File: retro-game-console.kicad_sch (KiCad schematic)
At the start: 16 parts, among them SW1 SW_Push, SW2 SW_Push, U1 ESP32-DevKitC, U2 Battery_shield_v3, U3 Micro_SD_card_adapter, U4 MAX98357A_Breakout, U5 LCD_ILI9341, U6 74HC165

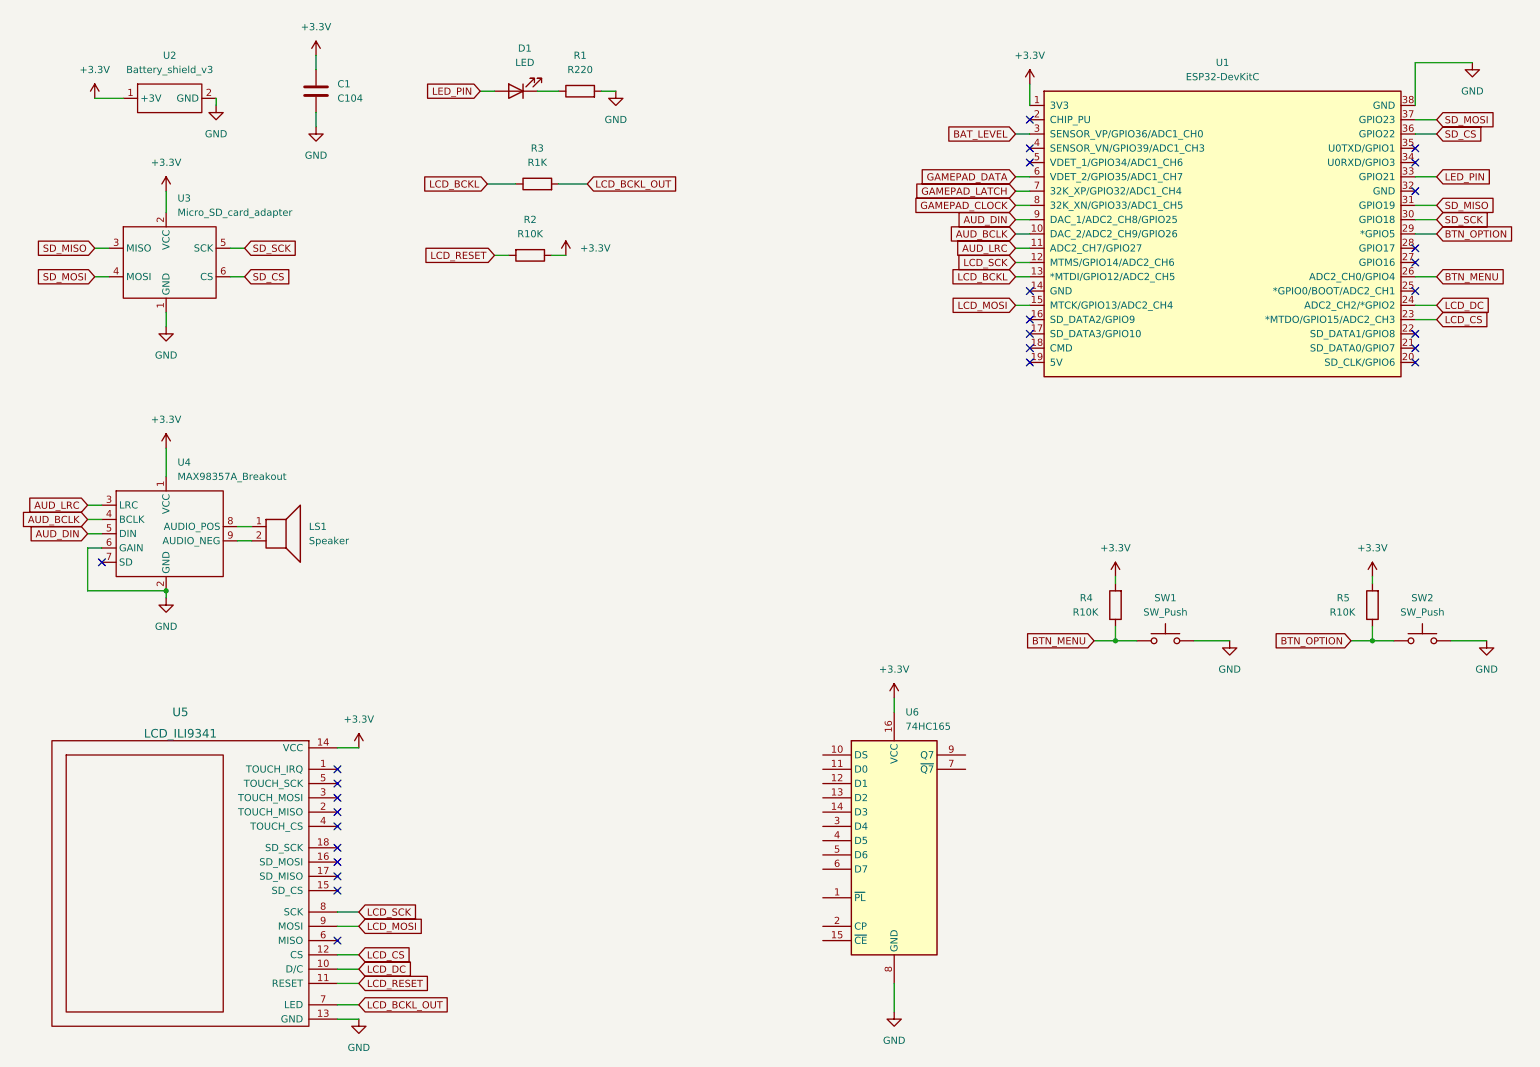
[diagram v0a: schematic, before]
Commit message: Schema done
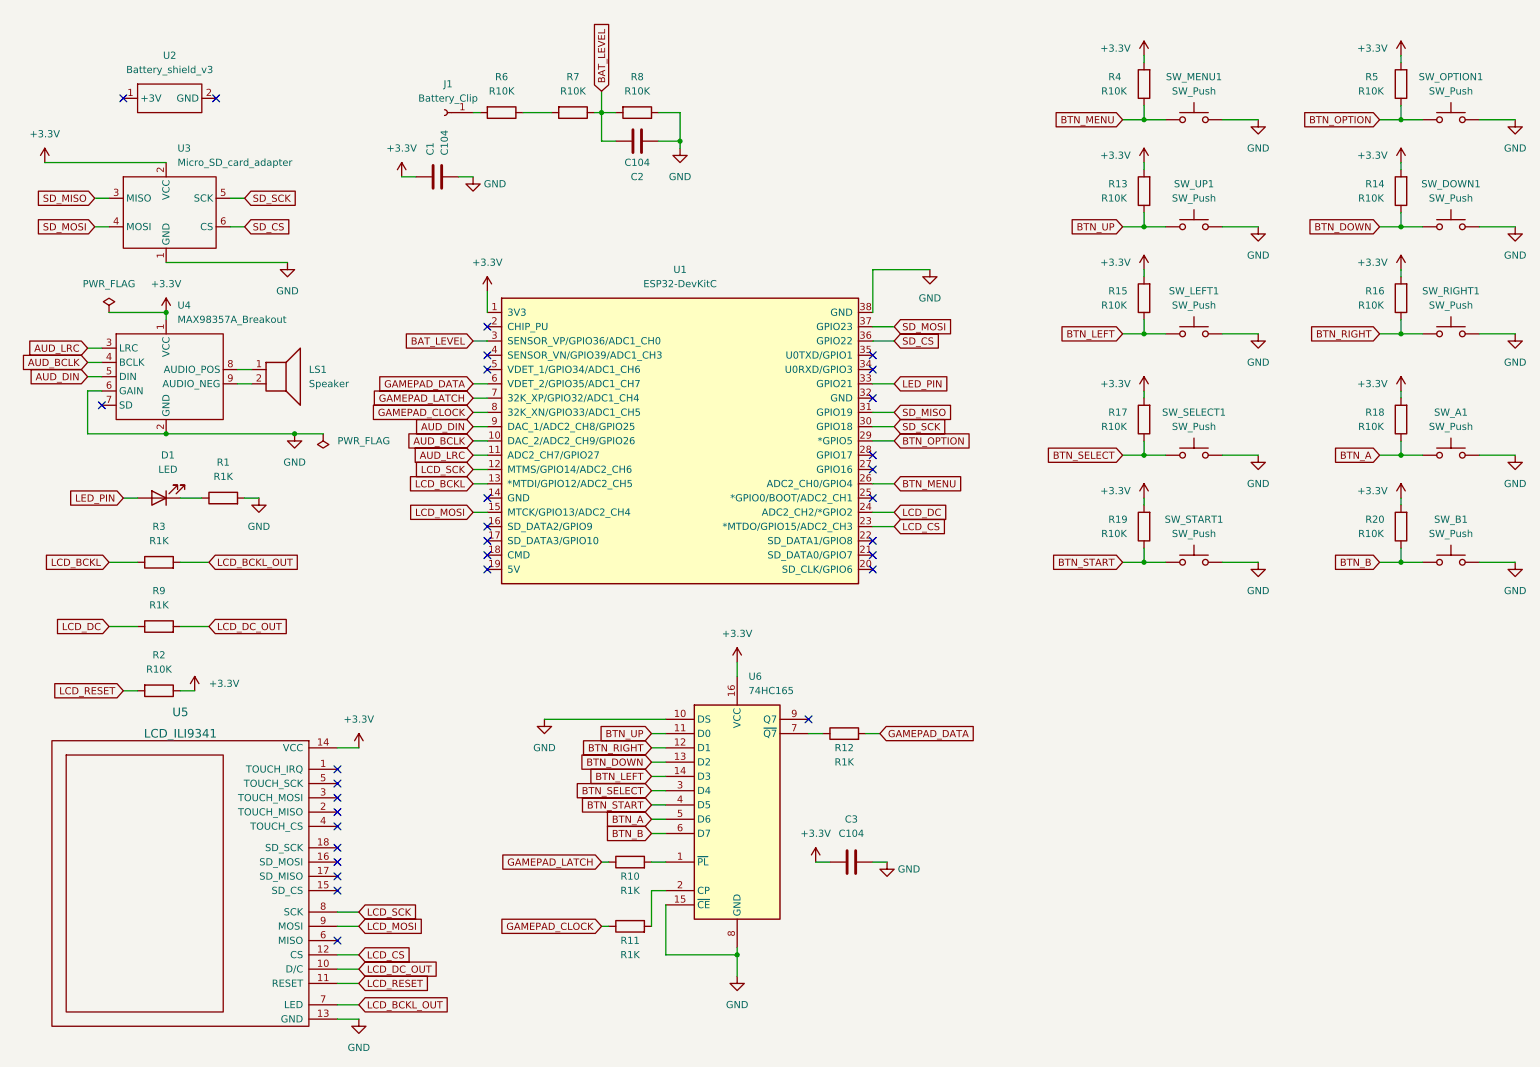
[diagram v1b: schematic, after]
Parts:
- added C2, C3: C104, Capacitor_THT:C_Rect_L7.0mm_W3.5mm_P5.00mm, symbol Device:C
- added J1: Battery_Clip, Connector_PinSocket_2.54mm:PinSocket_1x01_P2.54mm_Vertical, symbol Connector:Conn_01x01_Female
- added R10, R11, R12, R9: R1K, Resistor_THT:R_Axial_DIN0309_L9.0mm_D3.2mm_P12.70mm_Horizontal, symbol Device:R
- added R13, R14, R15, R16, R17, R18, R19, R20, R6, R7, R8: R10K, Resistor_THT:R_Axial_DIN0309_L9.0mm_D3.2mm_P12.70mm_Horizontal, symbol Device:R
- added SW_A1, SW_SELECT1, SW_START1: SW_Push, Button_Switch_SMD:SW_Push_1P1T_NO_6x6mm_H9.5mm, symbol Switch:SW_Push
- added SW_B1, SW_DOWN1, SW_LEFT1, SW_RIGHT1, SW_UP1: SW_Push, Button_Switch_THT:SW_PUSH-12mm, symbol Switch:SW_Push
- D1: footprint (none) -> LED_THT:LED_D5.0mm
- R1: value R220 -> R1K; footprint LED_THT:LED_D5.0mm -> Resistor_THT:R_Axial_DIN0309_L9.0mm_D3.2mm_P12.70mm_Horizontal
- R2, R4, R5: footprint LED_THT:LED_D5.0mm -> Resistor_THT:R_Axial_DIN0309_L9.0mm_D3.2mm_P12.70mm_Horizontal
- R3: footprint (none) -> Resistor_THT:R_Axial_DIN0309_L9.0mm_D3.2mm_P12.70mm_Horizontal
- SW_MENU1: renamed from SW1; footprint Button_Switch_THT:SW_PUSH_6mm_H5mm -> Button_Switch_SMD:SW_Push_1P1T_NO_6x6mm_H9.5mm
- SW_OPTION1: renamed from SW2; footprint Button_Switch_THT:SW_PUSH_6mm_H5mm -> Button_Switch_SMD:SW_Push_1P1T_NO_6x6mm_H9.5mm
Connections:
- net +3.3V: now also C3.2, R13.2, R14.2, R15.2, R16.2, R17.2, R18.2, R19.2, R20.2; no longer U2.1 (+3V)
- net BAT_LEVEL: now also C2.2, R7.1, R8.2
- net GAMEPAD_CLOCK: now also R11.1
- net GAMEPAD_DATA: now also R12.2
- net GAMEPAD_LATCH: now also R10.1
- net GND: now also U6.10 (DS), U6.15 (~{CE}), C2.1, C3.1, R8.1, SW_A1.2, SW_B1.2, SW_DOWN1.2, SW_LEFT1.2, SW_RIGHT1.2, SW_SELECT1.2, SW_START1.2, SW_UP1.2; no longer U2.2 (GND)
- net LCD_DC: now also R9.1; no longer U5.10 (D/C)
- net at U6.1 (~{PL}): now also R10.2
- net BTN_UP: now reaches U6.11 (D0)
- net BTN_UP: now also R13.1, SW_UP1.1
- net BTN_RIGHT: now reaches U6.12 (D1)
- net BTN_RIGHT: now also R16.1, SW_RIGHT1.1
- net BTN_DOWN: now reaches U6.13 (D2)
- net BTN_DOWN: now also R14.1, SW_DOWN1.1
- net BTN_LEFT: now reaches U6.14 (D3)
- net BTN_LEFT: now also R15.1, SW_LEFT1.1
- net at U6.2 (CP): now also R11.2
- net BTN_SELECT: now reaches U6.3 (D4)
- net BTN_SELECT: now also R17.1, SW_SELECT1.1
- net BTN_START: now reaches U6.4 (D5)
- net BTN_START: now also R19.1, SW_START1.1
- net BTN_A: now reaches U6.5 (D6)
- net BTN_A: now also R18.1, SW_A1.1
- net BTN_B: now reaches U6.6 (D7)
- net BTN_B: now also R20.1, SW_B1.1
- net at U6.7 (~{Q7}): now also R12.1
- new net: R6.1, R7.2
- new net: J1.1 (Pin_1), R6.2
- new net LCD_DC_OUT: R9.2, U5.10 (D/C)
- no-connect marks 28 -> 31
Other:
- moved on the sheet: C1, D1, LS1, R1, R2, R3, R4, R5, SW_MENU1, SW_OPTION1, U1, U3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
